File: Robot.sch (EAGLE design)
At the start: 7 parts, among them U1 LSM9DS0

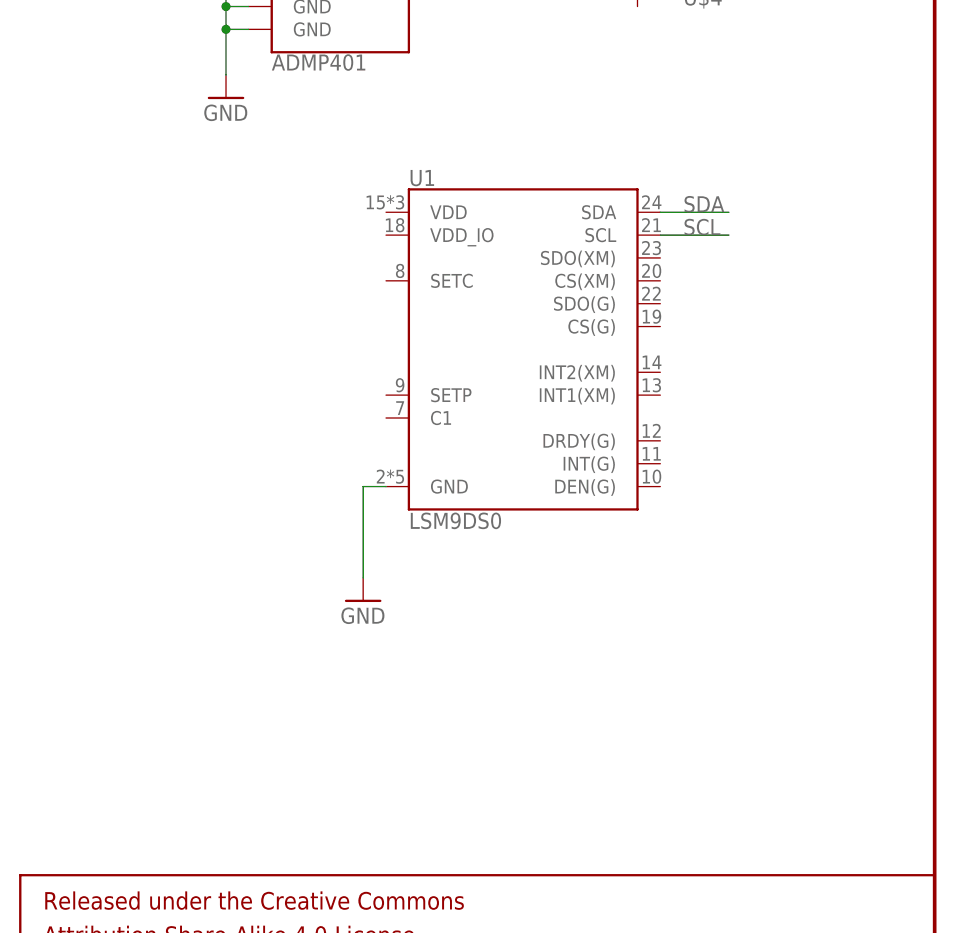
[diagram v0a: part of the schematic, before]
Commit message: Almost done with LSM9DS0
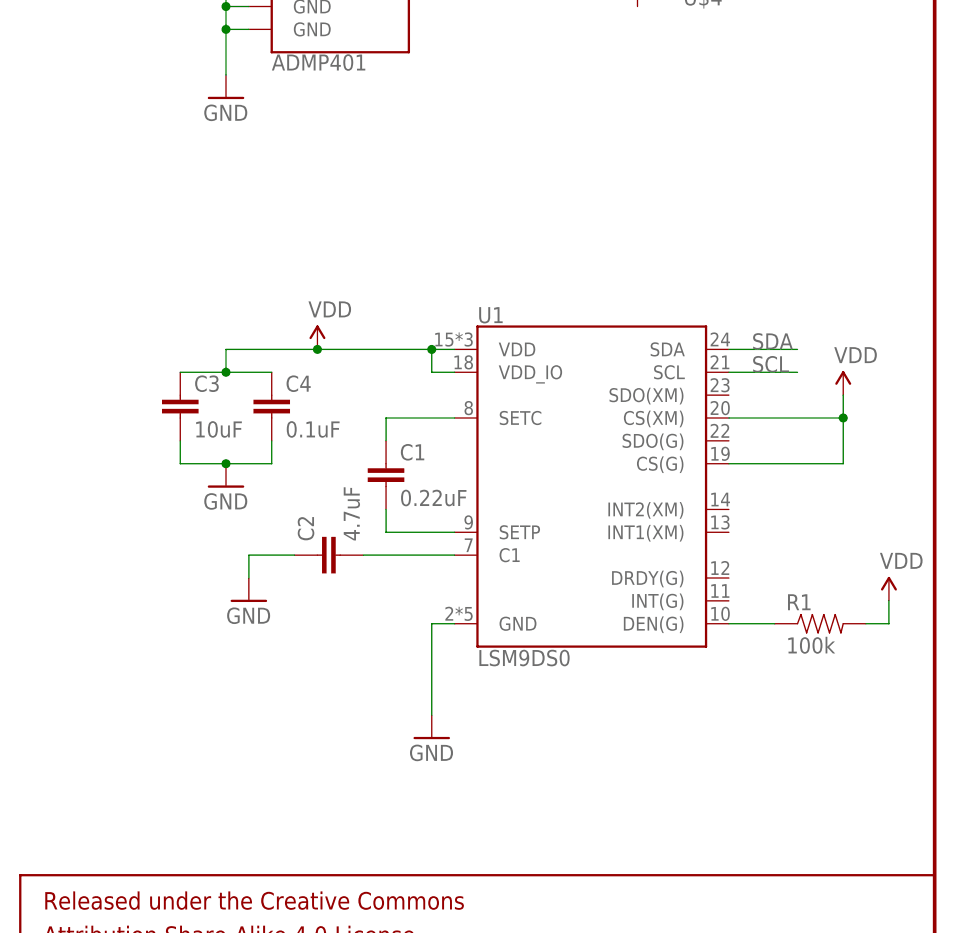
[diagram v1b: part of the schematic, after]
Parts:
- added C1: 0.22uF, SparkFun-Capacitors:0.22UF-25V-10%(0603)
- added C2: 4.7uF, SparkFun-Capacitors:4.7UF-6.3V-10%(0603)0603
- added C3: 10uF, SparkFun-Capacitors:10UF-6.3V-20%(0603)
- added C4: 0.1uF, SparkFun-Capacitors:0.1UF-100V-10%(0603)
- added R1: 100k, SparkFun-Resistors:100KOHM-1/10W-1%(0603)
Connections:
- new net N$1: C1.1, U1.SETC
- new net N$2: C1.2, U1.SETP
- new net N$3: C2.2, U1.C1
- new net N$4: R1.1, U1.DEN(G)
- new net VDD: C3.1, C4.1, R1.2, U1.CS(G), U1.CS(XM), U1.VDD, U1.VDD_IO
- net GND: now also C2.1, C3.2, C4.2
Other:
- moved on the sheet: U1
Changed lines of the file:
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@@
 <part name="U$4" library="SparkFun-AnalogIC" deviceset="MCP6291" device="T-E/OT"/>
 <part name="GND6" library="SparkFun-Aesthetics" deviceset="GND" device=""/>
+<part name="C1" library="SparkFun-Capacitors" deviceset="0.22UF-25V-10%(0603)" device="" value="0.22uF"/>
+<part name="C2" library="SparkFun-Capacitors" deviceset="4.7UF-6.3V-10%(0603)" device="0603" value="4.7uF"/>
+<part name="GND7" library="SparkFun-Aesthetics" deviceset="GND" device=""/>
+<part name="C3" library="SparkFun-Capacitors" deviceset="10UF-6.3V-20%(0603)" device="" value="10uF"/>
+<part name="C4" library="SparkFun-Capacitors" deviceset="0.1UF-100V-10%(0603)" device="" value="0.1uF"/>
+<part name="GND8" library="SparkFun-Aesthetics" deviceset="GND" device=""/>
+<part name="SUPPLY1" library="SparkFun-Aesthetics" deviceset="VDD" device=""/>
+<part name="R1" library="SparkFun-Resistors" deviceset="100KOHM-1/10W-1%(0603)" device="" value="100k"/>
+<part name="SUPPLY2" library="SparkFun-Aesthetics" deviceset="VDD" device=""/>
+<part name="SUPPLY3" library="SparkFun-Aesthetics" deviceset="VDD" device=""/>
 </parts>
 <sheets>
@@
 <instance part="U$2" gate="G$1" x="-7.62" y="2.54"/>
 <instance part="U$3" gate="G$1" x="86.36" y="134.62"/>
-<instance part="U1" gate="G$1" x="185.42" y="88.9"/>
-<instance part="GND1" gate="1" x="167.64" y="60.96"/>
+<instance part="U1" gate="G$1" x="193.04" y="73.66"/>
+<instance part="GND1" gate="1" x="175.26" y="45.72"/>
 <instance part="GND2" gate="1" x="63.5" y="43.18"/>
 <instance part="GND3" gate="1" x="40.64" y="165.1"/>
@@
 <instance part="U$4" gate="G$1" x="198.12" y="134.62"/>
 <instance part="GND6" gate="1" x="152.4" y="116.84"/>
+<instance part="C1" gate="G$1" x="170.18" y="73.66"/>
+<instance part="C2" gate="G$1" x="165.1" y="66.04" rot="R90"/>
+<instance part="GND7" gate="1" x="154.94" y="60.96"/>
+<instance part="C3" gate="G$1" x="147.32" y="81.28"/>
+<instance part="C4" gate="G$1" x="157.48" y="81.28"/>
+<instance part="GND8" gate="1" x="152.4" y="73.66"/>
+<instance part="SUPPLY1" gate="VDD" x="162.56" y="88.9"/>
+<instance part="R1" gate="G$1" x="218.44" y="58.42"/>
+<instance part="SUPPLY2" gate="VDD" x="226.06" y="60.96"/>
+<instance part="SUPPLY3" gate="VDD" x="220.98" y="83.82"/>
 </instances>
 <busses>
@@
 <segment>
 <pinref part="U1" gate="G$1" pin="SDA"/>
-<wire x1="208.28" y1="104.14" x2="200.66" y2="104.14" width="0.1524" layer="91"/>
-<label x="203.2" y="104.14" size="1.778" layer="95"/>
+<wire x1="215.9" y1="88.9" x2="208.28" y2="88.9" width="0.1524" layer="91"/>
+<label x="210.82" y="88.9" size="1.778" layer="95"/>
 </segment>
 <segment>
@@
 <segment>
 <pinref part="U1" gate="G$1" pin="SCL"/>
-<wire x1="208.28" y1="101.6" x2="200.66" y2="101.6" width="0.1524" layer="91"/>
-<label x="203.2" y="101.6" size="1.778" layer="95"/>
+<wire x1="215.9" y1="86.36" x2="208.28" y2="86.36" width="0.1524" layer="91"/>
+<label x="210.82" y="86.36" size="1.778" layer="95"/>
 </segment>
 <segment>
@@
 <segment>
 <pinref part="GND1" gate="1" pin="GND"/>
-<wire x1="167.64" y1="63.5" x2="167.64" y2="73.66" width="0.1524" layer="91"/>
+<wire x1="175.26" y1="48.26" x2="175.26" y2="58.42" width="0.1524" layer="91"/>
 <pinref part="U1" gate="G$1" pin="GND"/>
-<wire x1="167.64" y1="73.66" x2="170.18" y2="73.66" width="0.1524" layer="91"/>
+<wire x1="175.26" y1="58.42" x2="177.8" y2="58.42" width="0.1524" layer="91"/>
 </segment>
 <segment>
@@
 <junction x="152.4" y="124.46"/>
 </segment>
+<segment>
+<pinref part="GND7" gate="1" pin="GND"/>
+<wire x1="154.94" y1="63.5" x2="154.94" y2="66.04" width="0.1524" layer="91"/>
+<pinref part="C2" gate="G$1" pin="1"/>
+<wire x1="154.94" y1="66.04" x2="160.02" y2="66.04" width="0.1524" layer="91"/>
+</segment>
+<segment>
+<pinref part="C3" gate="G$1" pin="2"/>
+<wire x1="147.32" y1="78.74" x2="147.32" y2="76.2" width="0.1524" layer="91"/>
+<pinref part="GND8" gate="1" pin="GND"/>
+<wire x1="147.32" y1="76.2" x2="152.4" y2="76.2" width="0.1524" layer="91"/>
+<pinref part="C4" gate="G$1" pin="2"/>
+<wire x1="157.48" y1="78.74" x2="157.48" y2="76.2" width="0.1524" layer="91"/>
+<wire x1="157.48" y1="76.2" x2="152.4" y2="76.2" width="0.1524" layer="91"/>
+<junction x="152.4" y="76.2"/>
+</segment>
 </net>
 <net name="MOTOR1" class="0">
@@
 </segment>
 </net>
+<net name="N$1" class="0">
+<segment>
+<pinref part="C1" gate="G$1" pin="1"/>
+<wire x1="170.18" y1="78.74" x2="170.18" y2="81.28" width="0.1524" layer="91"/>
+<pinref part="U1" gate="G$1" pin="SETC"/>
+<wire x1="170.18" y1="81.28" x2="177.8" y2="81.28" width="0.1524" layer="91"/>
+</segment>
+</net>
+<net name="N$2" class="0">
+<segment>
+<pinref part="C1" gate="G$1" pin="2"/>
+<wire x1="170.18" y1="71.12" x2="170.18" y2="68.58" width="0.1524" layer="91"/>
+<pinref part="U1" gate="G$1" pin="SETP"/>
+<wire x1="170.18" y1="68.58" x2="177.8" y2="68.58" width="0.1524" layer="91"/>
+</segment>
+</net>
+<net name="N$3" class="0">
+<segment>
+<pinref part="C2" gate="G$1" pin="2"/>
+<pinref part="U1" gate="G$1" pin="C1"/>
+<wire x1="167.64" y1="66.04" x2="177.8" y2="66.04" width="0.1524" layer="91"/>
+</segment>
+</net>
+<net name="VDD" class="0">
+<segment>
+<pinref part="C3" gate="G$1" pin="1"/>
+<pinref part="C4" gate="G$1" pin="1"/>
+<wire x1="147.32" y1="86.36" x2="152.4" y2="86.36" width="0.1524" layer="91"/>
+<wire x1="152.4" y1="86.36" x2="157.48" y2="86.36" width="0.1524" layer="91"/>
+<wire x1="152.4" y1="86.36" x2="152.4" y2="88.9" width="0.1524" layer="91"/>
+<junction x="152.4" y="86.36"/>
+<pinref part="U1" gate="G$1" pin="VDD"/>
+<wire x1="152.4" y1="88.9" x2="162.56" y2="88.9" width="0.1524" layer="91"/>
+<wire x1="162.56" y1="88.9" x2="175.26" y2="88.9" width="0.1524" layer="91"/>
+<pinref part="SUPPLY1" gate="VDD" pin="VDD"/>
+<junction x="162.56" y="88.9"/>
+<pinref part="U1" gate="G$1" pin="VDD_IO"/>
+<wire x1="175.26" y1="88.9" x2="177.8" y2="88.9" width="0.1524" layer="91"/>
+<wire x1="177.8" y1="86.36" x2="175.26" y2="86.36" width="0.1524" layer="91"/>
+<wire x1="175.26" y1="86.36" x2="175.26" y2="88.9" width="0.1524" layer="91"/>
+<junction x="175.26" y="88.9"/>
+</segment>
+<segment>
+<pinref part="R1" gate="G$1" pin="2"/>
+<pinref part="SUPPLY2" gate="VDD" pin="VDD"/>
+<wire x1="223.52" y1="58.42" x2="226.06" y2="58.42" width="0.1524" layer="91"/>
+<wire x1="226.06" y1="58.42" x2="226.06" y2="60.96" width="0.1524" layer="91"/>
+</segment>
+<segment>
+<pinref part="U1" gate="G$1" pin="CS(XM)"/>
+<pinref part="SUPPLY3" gate="VDD" pin="VDD"/>
+<wire x1="208.28" y1="81.28" x2="220.98" y2="81.28" width="0.1524" layer="91"/>
+<wire x1="220.98" y1="81.28" x2="220.98" y2="83.82" width="0.1524" layer="91"/>
+<pinref part="U1" gate="G$1" pin="CS(G)"/>
+<wire x1="208.28" y1="76.2" x2="220.98" y2="76.2" width="0.1524" layer="91"/>
+<wire x1="220.98" y1="76.2" x2="220.98" y2="81.28" width="0.1524" layer="91"/>
+<junction x="220.98" y="81.28"/>
+</segment>
+</net>
+<net name="N$4" class="0">
+<segment>
+<pinref part="U1" gate="G$1" pin="DEN(G)"/>
+<pinref part="R1" gate="G$1" pin="1"/>
+<wire x1="208.28" y1="58.42" x2="213.36" y2="58.42" width="0.1524" layer="91"/>
+</segment>
+</net>

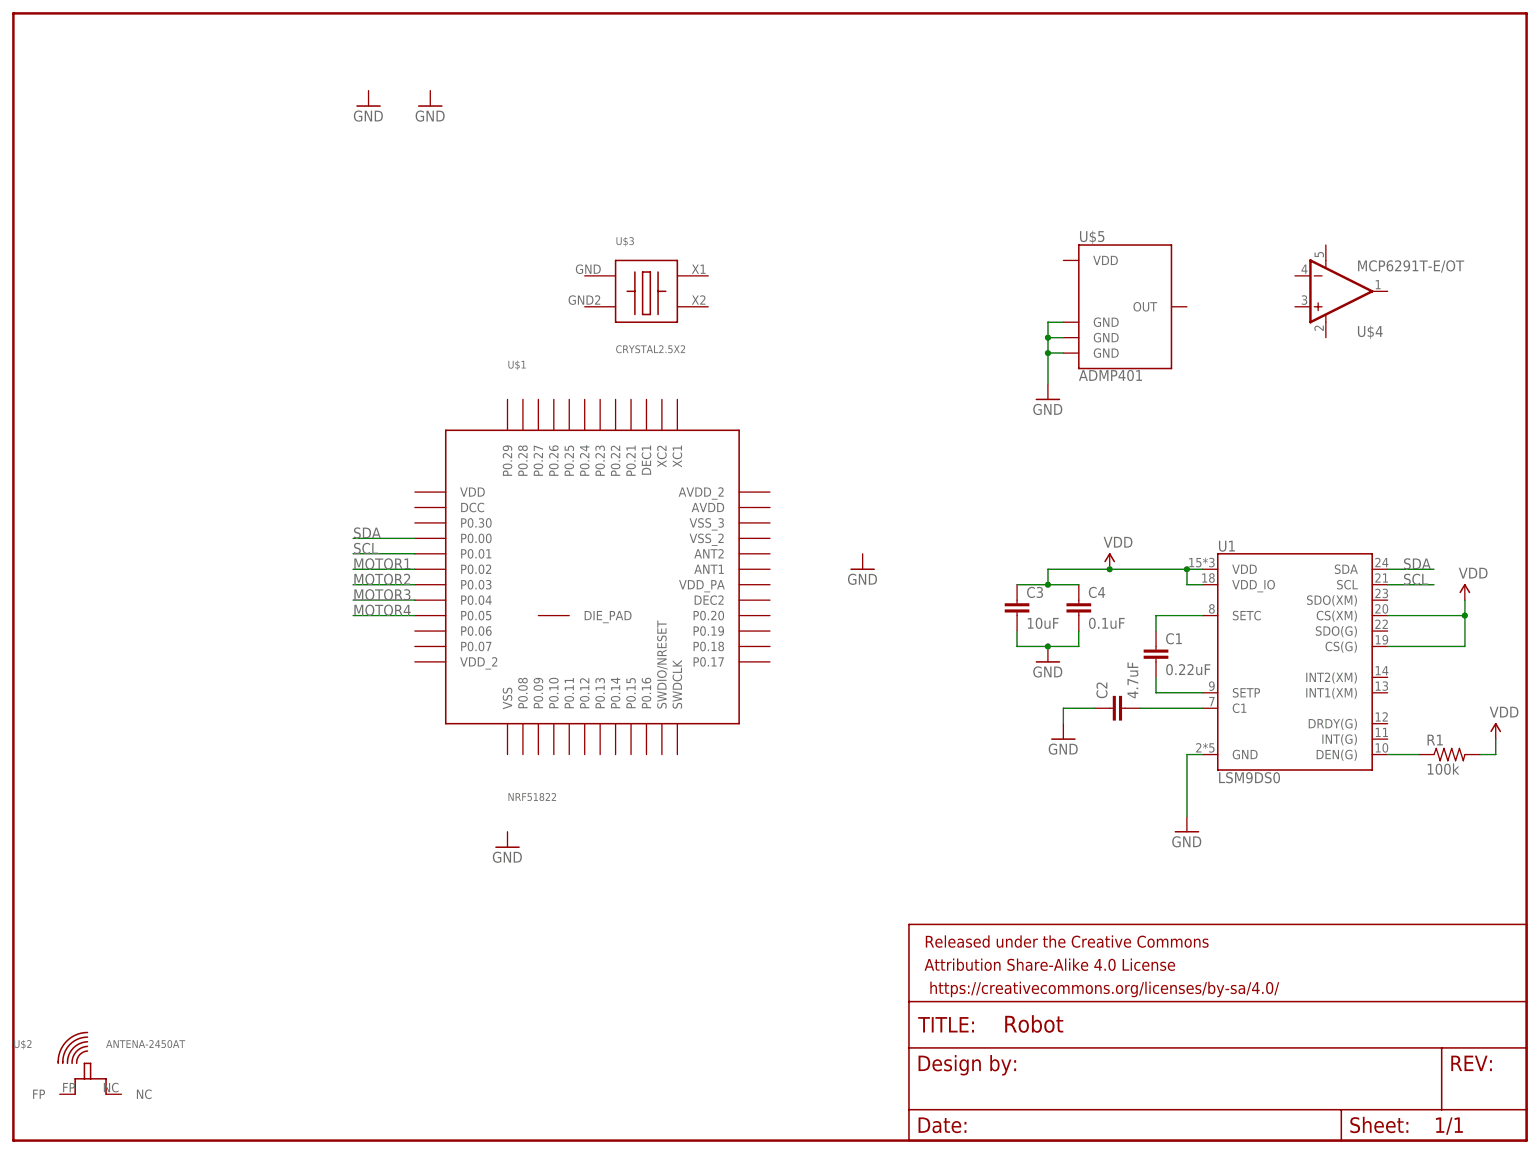
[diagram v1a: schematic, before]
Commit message: did some routing
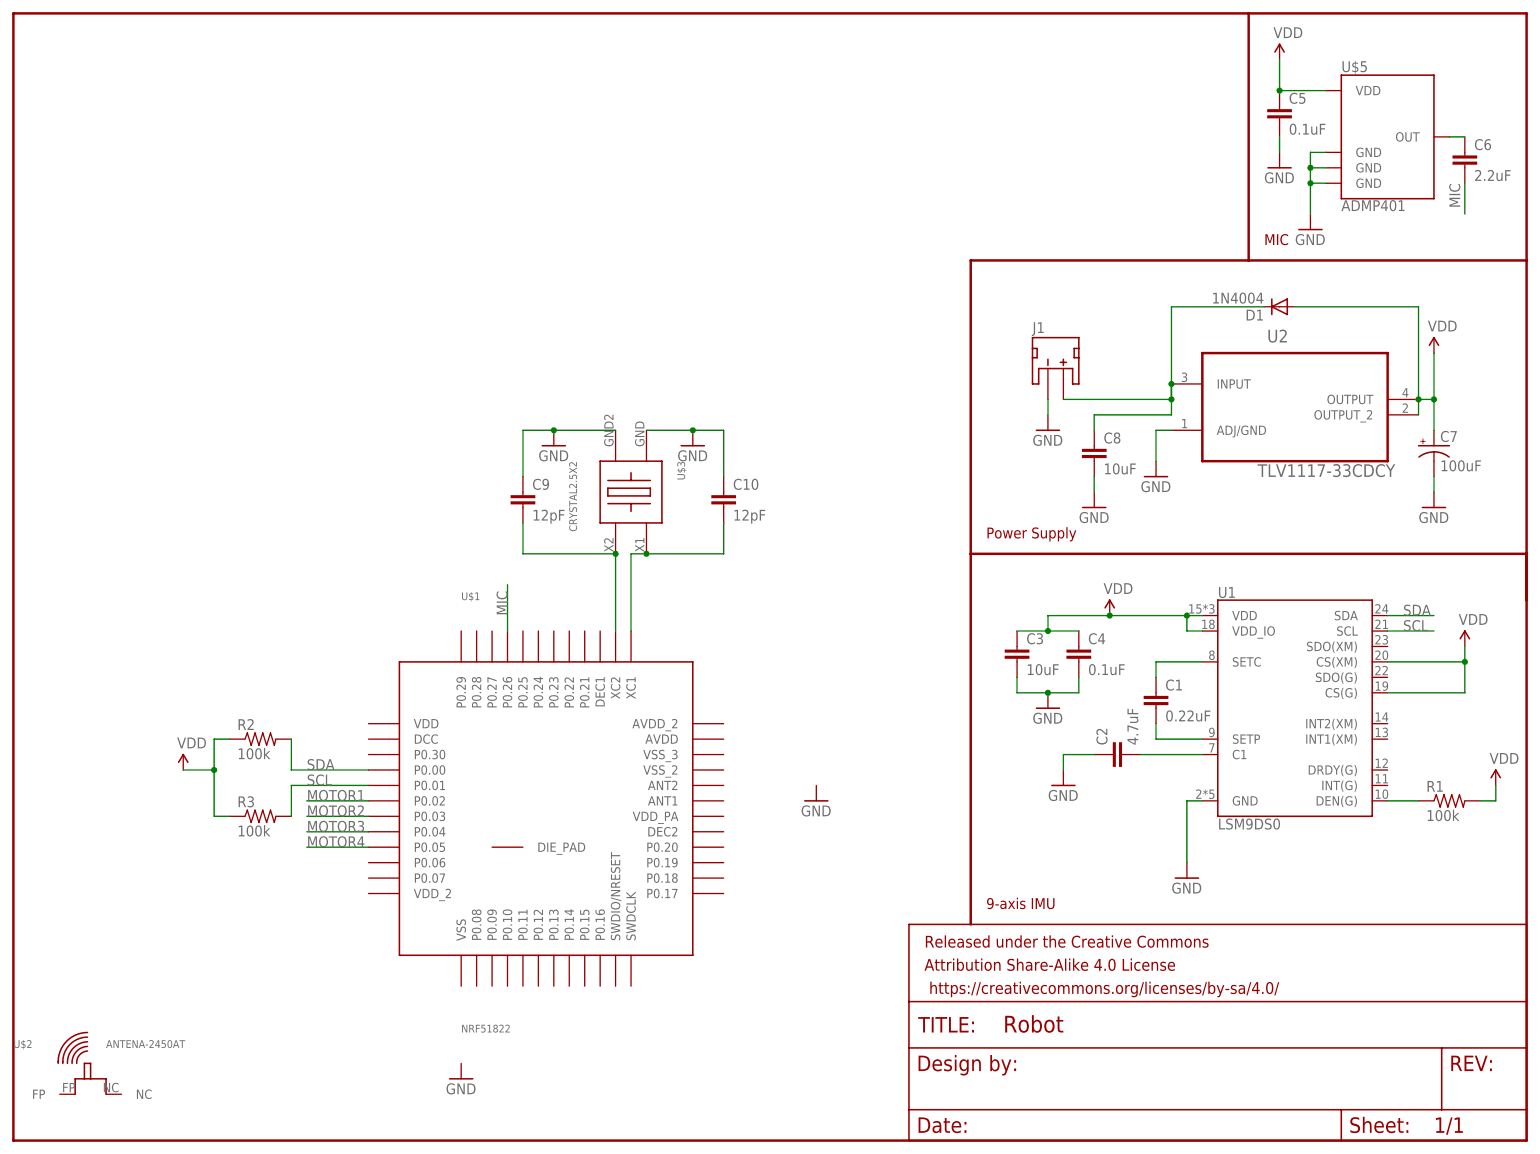
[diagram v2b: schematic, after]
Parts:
- removed U$4: MCP6291T-E/OT, SparkFun-AnalogIC:MCP6291T-E/OT
- added C10, C9: 12pF, SparkFun-Capacitors:12PF-50V-5%(0603)
- added C5: 0.1uF, SparkFun-Capacitors:0.1UF-100V-10%(0603)
- added C6: 2.2uF, SparkFun-Capacitors:2.2UF-10V-20%(0603)
- added C7: 100uF, SparkFun-Capacitors:100UF-10V-10%(TANT)
- added C8: 10uF, SparkFun-Capacitors:10UF-6.3V-20%(0603)
- added D1: 1N4004, diode:1N4004
- added J1: (no value), SparkFun-Connectors:JST_2MM_MALE
- added R2, R3: 100k, SparkFun-Resistors:100KOHM-1/10W-1%(0603)
- added U2: TLV1117-33CDCY, Texas Instruments_By_element14_Batch_1:TLV1117-33CDCY
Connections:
- new net MIC: C6.2, U$1.P0.26
- new net N$5: C8.1, D1.C, J1.+, U2.INPUT
- new net N$6: C6.1, U$5.OUT
- new net N$8: C9.2, U$1.XC2, U$3.X2
- new net N$9: C10.2, U$1.XC1, U$3.X1
- net GND: now also C10.1, C5.2, C7.-, C8.2, C9.1, J1.-, U$3.GND, U$3.GND2, U2.ADJ/GND
- net SCL: now also R3.2
- net SDA: now also R2.2
- net VDD: now also C5.1, C7.+, D1.A, R2.1, R3.1, U$5.VDD, U2.OUTPUT, U2.OUTPUT_2
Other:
- note added: "9-axis IMU"
- note added: "MIC"
- note added: "Power Supply"
- moved on the sheet: C1, C2, C3, C4, R1, U$1, U$3, U$5, U1
